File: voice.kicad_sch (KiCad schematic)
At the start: 14 parts, among them U2 AP2112K-3.3, U3 WM8960CGEFL_V, Y1 ECS-3225MV

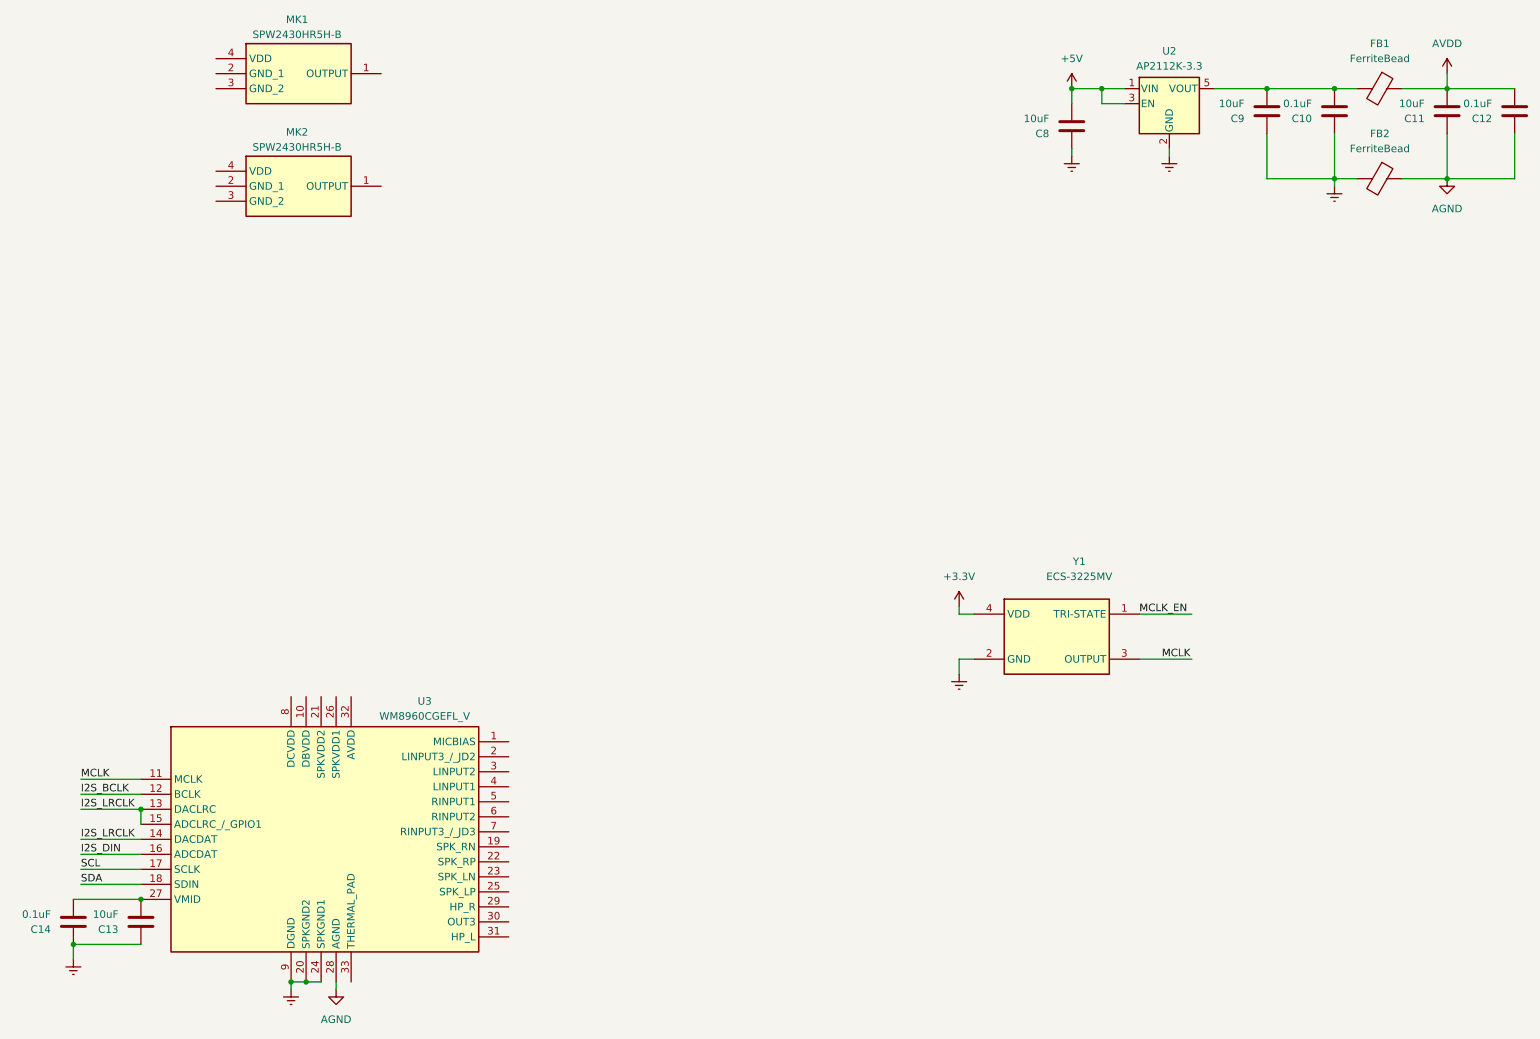
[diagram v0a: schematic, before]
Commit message: voice schematic
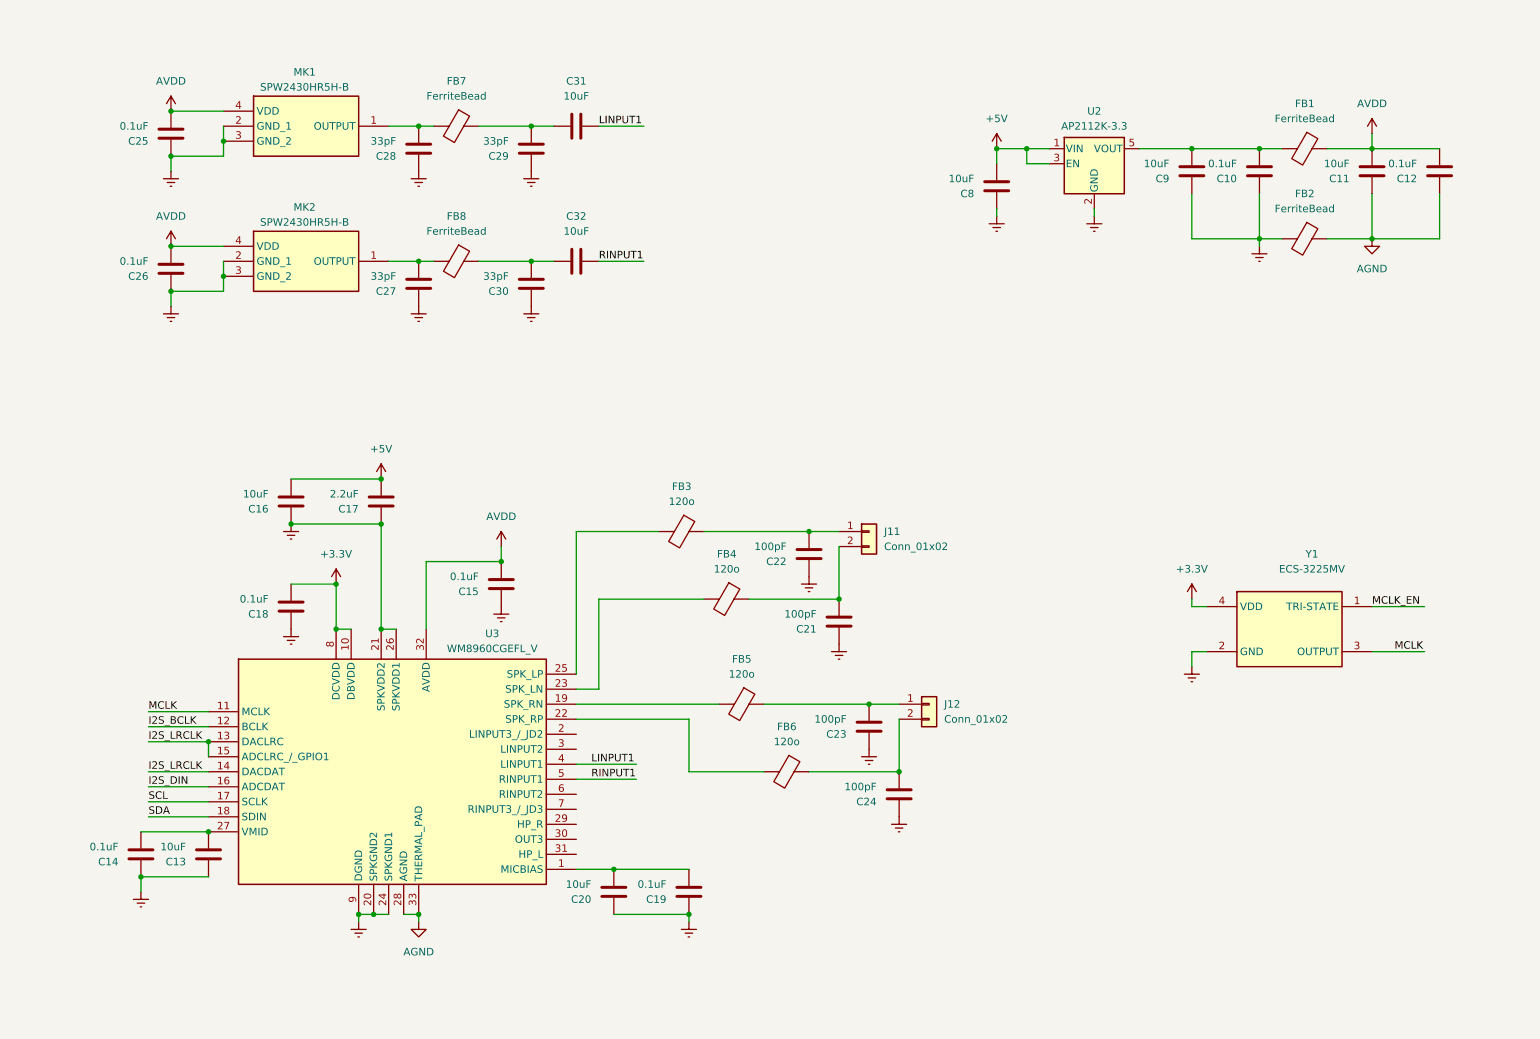
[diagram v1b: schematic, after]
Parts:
- added C15, C18, C19, C25, C26: 0.1uF, Capacitor_SMD:C_0603_1608Metric_Pad1.08x0.95mm_HandSolder, symbol Device:C
- added C16, C20, C31, C32: 10uF, Capacitor_SMD:C_0603_1608Metric_Pad1.08x0.95mm_HandSolder, symbol Device:C
- added C17: 2.2uF, Capacitor_SMD:C_0603_1608Metric_Pad1.08x0.95mm_HandSolder, symbol Device:C
- added C21, C22, C23, C24: 100pF, Capacitor_SMD:C_0603_1608Metric_Pad1.08x0.95mm_HandSolder, symbol Device:C
- added C27, C28, C29, C30: 33pF, Capacitor_SMD:C_0603_1608Metric_Pad1.08x0.95mm_HandSolder, symbol Device:C
- added FB3, FB4, FB5, FB6: 120o, Inductor_SMD:L_0603_1608Metric_Pad1.05x0.95mm_HandSolder, symbol Device:FerriteBead
- added FB7, FB8: FerriteBead, Inductor_SMD:L_0603_1608Metric_Pad1.05x0.95mm_HandSolder, symbol Device:FerriteBead
- added J11, J12: Conn_01x02, Connector_PinHeader_2.54mm:PinHeader_1x02_P2.54mm_Vertical, symbol Connector_Generic:Conn_01x02
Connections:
- net +3.3V: now also U3.10 (DBVDD), U3.8 (DCVDD), C18.2
- net +5V: now also C16.2, C17.2
- net AGND: now also U3.33 (THERMAL_PAD)
- net AVDD: now also MK1.4 (VDD), MK2.4 (VDD), U3.32 (AVDD), C15.2, C25.2, C26.2
- net Earth: now also MK1.2 (GND_1), MK1.3 (GND_2), MK2.2 (GND_1), MK2.3 (GND_2), U3.21 (SPKVDD2), U3.26 (SPKVDD1), C15.1, C16.1, C17.1, C18.1, C19.1, C20.1, C21.1, C22.1, C23.1, C24.1, C25.1, C26.1, C27.1, C28.1, C29.1, C30.1
- net at U3.1 (MICBIAS): now also C19.2, C20.2
- net at U3.19 (SPK_RN): now also FB5.2
- net at U3.22 (SPK_RP): now also FB6.2
- net at U3.23 (SPK_LN): now also FB4.2
- net at U3.25 (SPK_LP): now also FB3.2
- net LINPUT1: now reaches U3.4 (LINPUT1)
- net LINPUT1: now also C31.1
- net RINPUT1: now reaches U3.5 (RINPUT1)
- net RINPUT1: now also C32.1
- net at MK2.1 (OUTPUT): now also C27.2, FB8.2
- net at MK1.1 (OUTPUT): now also C28.2, FB7.2
- new net: C21.2, FB4.1, J11.2 (Pin_2)
- new net: C24.2, FB6.1, J12.2 (Pin_2)
- new net: C22.2, FB3.1, J11.1 (Pin_1)
- new net: C30.2, C32.2, FB8.1
- new net: C29.2, C31.2, FB7.1
- new net: C23.2, FB5.1, J12.1 (Pin_1)
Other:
- moved on the sheet: C10, C11, C12, C13, C14, C8, C9, FB1, FB2, MK1, MK2, U2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
